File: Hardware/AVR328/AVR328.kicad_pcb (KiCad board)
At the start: 2 copper layers, 58.5 x 56.9 mm, 33 parts, among them J1 EJ508A, J2 284512-8, J3 284512-8, Q2 S9013, Q3 S9013, Q4 S9013, Q5 S9013, U1 ATMEGA328P-AU, U2 L78M05CDT, Y1 Crystal

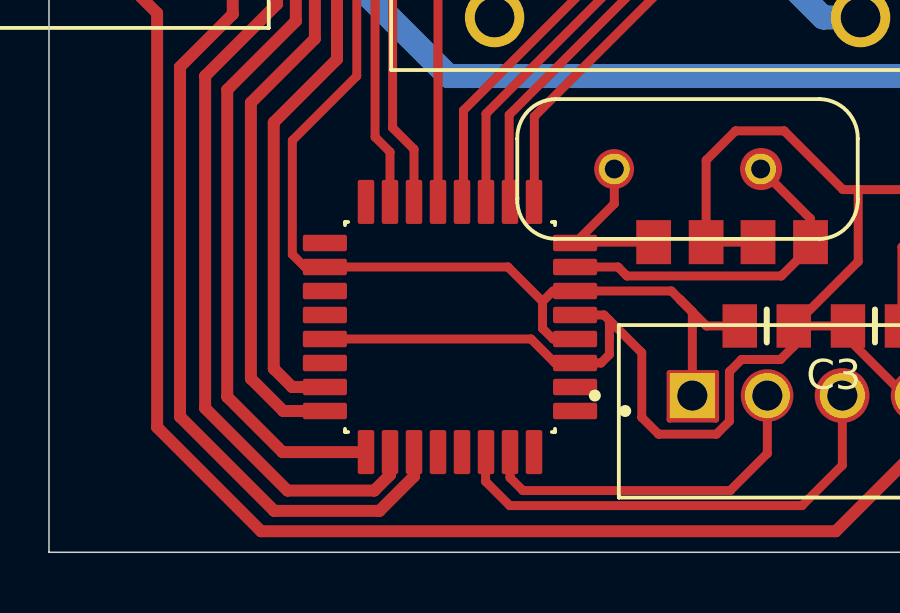
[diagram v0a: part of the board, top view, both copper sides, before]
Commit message: add
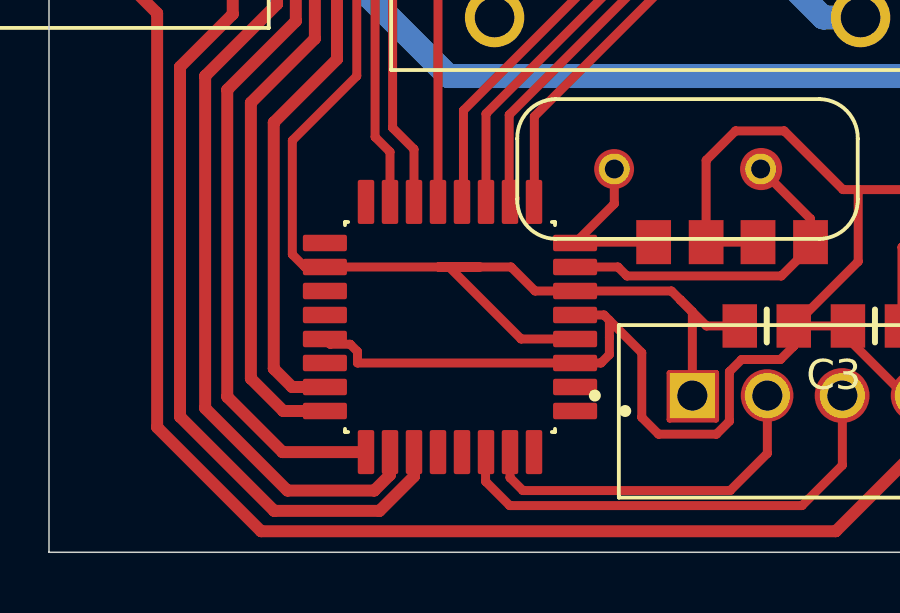
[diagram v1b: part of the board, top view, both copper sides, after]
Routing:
- net 5V: track 193.3 -> 197.5 mm
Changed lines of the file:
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@@
 		(tenting front back)
 		(pcbplotparams
-			(layerselection 0x00000000_00000000_55555555_555555f0)
+			(layerselection 0x00000000_00000000_55555555_55555554)
 			(plot_on_all_layers_selection 0x00000000_00000000_00000000_02000000)
 			(disableapertmacros no)
@@
 			(subtractmaskfromsilk no)
 			(outputformat 4)
-			(mirror no)
+			(mirror yes)
 			(drillshape 0)
 			(scaleselection 1)
@@
 	)
 	(segment
-		(start 73.931778 94.4652)
-		(end 74.731778 95.2652)
-		(width 0.3)
-		(layer "F.Cu")
-		(net 1)
-	)
-	(segment
 		(start 59.7017 81.8388)
 		(end 61.468 83.6051)
@@
 	)
 	(segment
+		(start 68.1458 95.2652)
+		(end 75.3998 95.2652)
+		(width 0.3)
+		(layer "F.Cu")
+		(net 1)
+	)
+	(segment
 		(start 100.2507 89.4854)
 		(end 100.47 89.7047)
@@
 	)
 	(segment
+		(start 67.901822 94.6392)
+		(end 68.1458 94.883178)
+		(width 0.3)
+		(layer "F.Cu")
+		(net 1)
+	)
+	(segment
 		(start 84.3292 89.4854)
 		(end 82.3722 87.5284)
@@
 	)
 	(segment
-		(start 67.0598 94.4652)
-		(end 73.931778 94.4652)
-		(width 0.3)
-		(layer "F.Cu")
-		(net 1)
-	)
-	(segment
 		(start 94.2848 89.4854)
 		(end 94.2848 89.4588)
@@
 	)
 	(segment
-		(start 75.3998 93.6652)
-		(end 76.365 93.6652)
+		(start 67.0598 94.4652)
+		(end 67.2338 94.6392)
 		(width 0.3)
 		(layer "F.Cu")
@@
 	)
 	(segment
-		(start 94.2848 89.4854)
-		(end 100.2507 89.4854)
+		(start 75.3998 93.6652)
+		(end 76.365 93.6652)
 		(width 0.3)
 		(layer "F.Cu")
@@
 	)
 	(segment
-		(start 74.731778 95.2652)
-		(end 75.3998 95.2652)
+		(start 94.2848 89.4854)
+		(end 100.2507 89.4854)
 		(width 0.3)
 		(layer "F.Cu")
@@
 	)
 	(segment
+		(start 68.1458 94.883178)
+		(end 68.1458 95.2652)
+		(width 0.3)
+		(layer "F.Cu")
+		(net 1)
+	)
+	(segment
 		(start 95.9612 64.8028)
 		(end 95.9612 53.6956)
@@
 	)
 	(segment
+		(start 67.2338 94.6392)
+		(end 67.901822 94.6392)
+		(width 0.3)
+		(layer "F.Cu")
+		(net 1)
+	)
+	(segment
 		(start 76.8288 92.0652)
 		(end 77.1278 92.3642)
@@
 	)
 	(segment
-		(start 73.1628 92.0652)
-		(end 74.3138 93.2162)
-		(width 0.3)
-		(layer "F.Cu")
-		(net 5)
-	)
-	(segment
 		(start 72.7162 71.7494)
 		(end 74.6196 71.7494)
@@
 	)
 	(segment
+		(start 67.0598 92.0652)
+		(end 70.85 92.0652)
+		(width 0.3)
+		(layer "F.Cu")
+		(net 5)
+	)
+	(segment
+		(start 74.0652 92.8652)
+		(end 75.3998 92.8652)
+		(width 0.3)
+		(layer "F.Cu")
+		(net 5)
+	)
+	(segment
 		(start 107.1118 72.3392)
 		(end 107.1118 65.2526)
@@
 	)
 	(segment
+		(start 73.2652 92.0652)
+		(end 74.0652 92.8652)
+		(width 0.3)
+		(layer "F.Cu")
+		(net 5)
+	)
+	(segment
 		(start 62.6812 55.632)
 		(end 72.7314 55.632)
@@
 	)
 	(segment
+		(start 73.6 94.4652)
+		(end 71.2 92.0652)
+		(width 0.3)
+		(layer "F.Cu")
+		(net 5)
+	)
+	(segment
 		(start 72.7314 55.632)
 		(end 74.4668 55.632)
@@
 	)
 	(segment
-		(start 74.6648 94.4652)
-		(end 75.3998 94.4652)
+		(start 75.3998 94.4652)
+		(end 73.6 94.4652)
 		(width 0.3)
 		(layer "F.Cu")
@@
 	)
 	(segment
-		(start 74.6648 92.8652)
-		(end 74.3138 93.2162)
-		(width 0.3)
-		(layer "F.Cu")
-		(net 5)
-	)
-	(segment
 		(start 104.5835 83.7494)
 		(end 103.9114 83.0773)
@@
 	)
 	(segment
-		(start 74.3138 93.2162)
-		(end 74.3138 94.1142)
+		(start 107.1118 65.2526)
+		(end 104.0638 62.2046)
 		(width 0.3)
 		(layer "F.Cu")
@@
 	)
 	(segment
-		(start 107.1118 65.2526)
-		(end 104.0638 62.2046)
+		(start 72.240298 92.0652)
+		(end 70.85 92.0652)
 		(width 0.3)
 		(layer "F.Cu")
@@
 	)
 	(segment
-		(start 75.3998 92.8652)
-		(end 74.6648 92.8652)
-		(width 0.3)
-		(layer "F.Cu")
-		(net 5)
-	)
-	(segment
 		(start 65.9738 87.8486)
 		(end 68.1228 85.6996)
@@
 	)
 	(segment
-		(start 74.3138 94.1142)
-		(end 74.6648 94.4652)
-		(width 0.3)
-		(layer "F.Cu")
-		(net 5)
-	)
-	(segment
 		(start 78.9037 93.1559)
 		(end 78.613 92.8652)
@@
 	)
 	(segment
-		(start 67.0598 92.0652)
-		(end 73.1628 92.0652)
+		(start 106.3752 54.356)
+		(end 105.918 53.8988)
 		(width 0.3)
 		(layer "F.Cu")
@@
 	)
 	(segment
-		(start 106.3752 54.356)
-		(end 105.918 53.8988)
+		(start 71.2 92.0652)
+		(end 73.2652 92.0652)
 		(width 0.3)
 		(layer "F.Cu")
@@
 		(layer "F.Cu")
 		(net 5)
+	)
+	(segment
+		(start 70.85 92.0652)
+		(end 71.2 92.0652)
+		(width 0.3)
+		(layer "F.Cu")
+		(net 5)

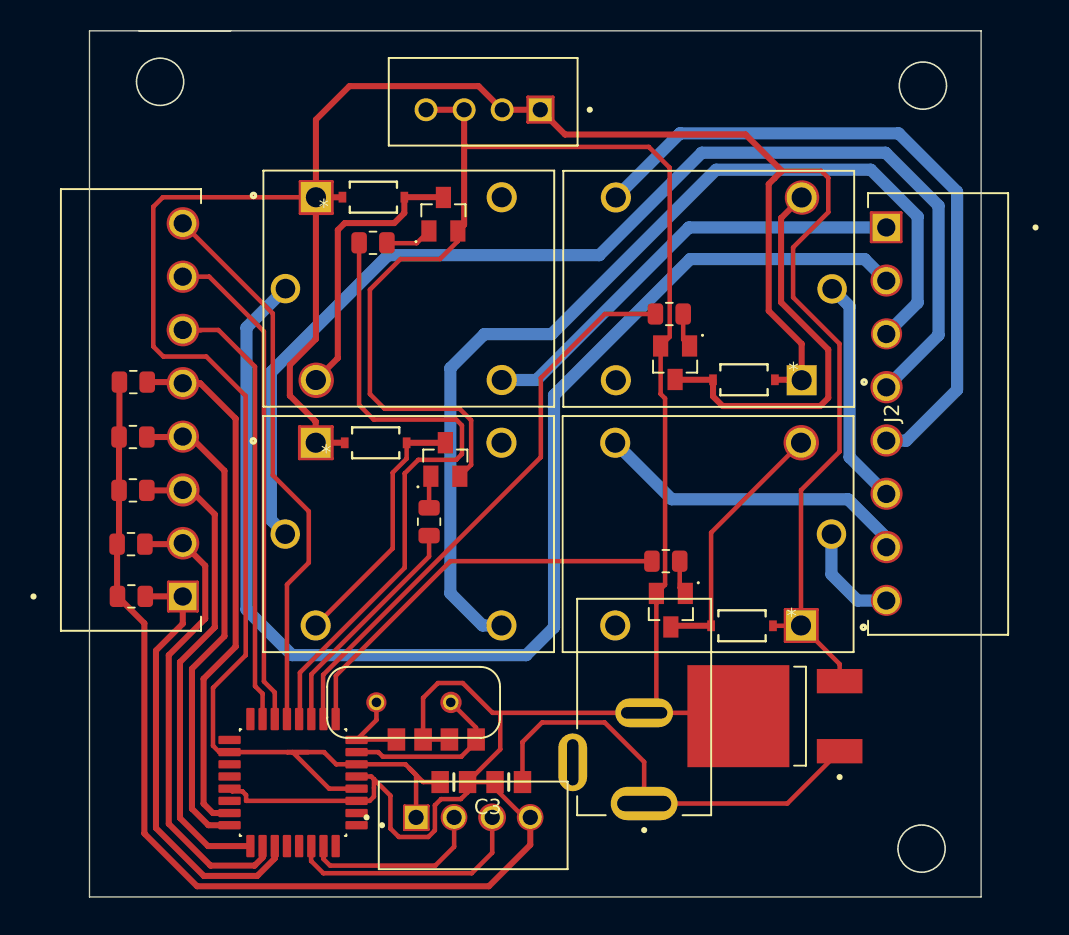
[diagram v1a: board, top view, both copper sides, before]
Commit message: add
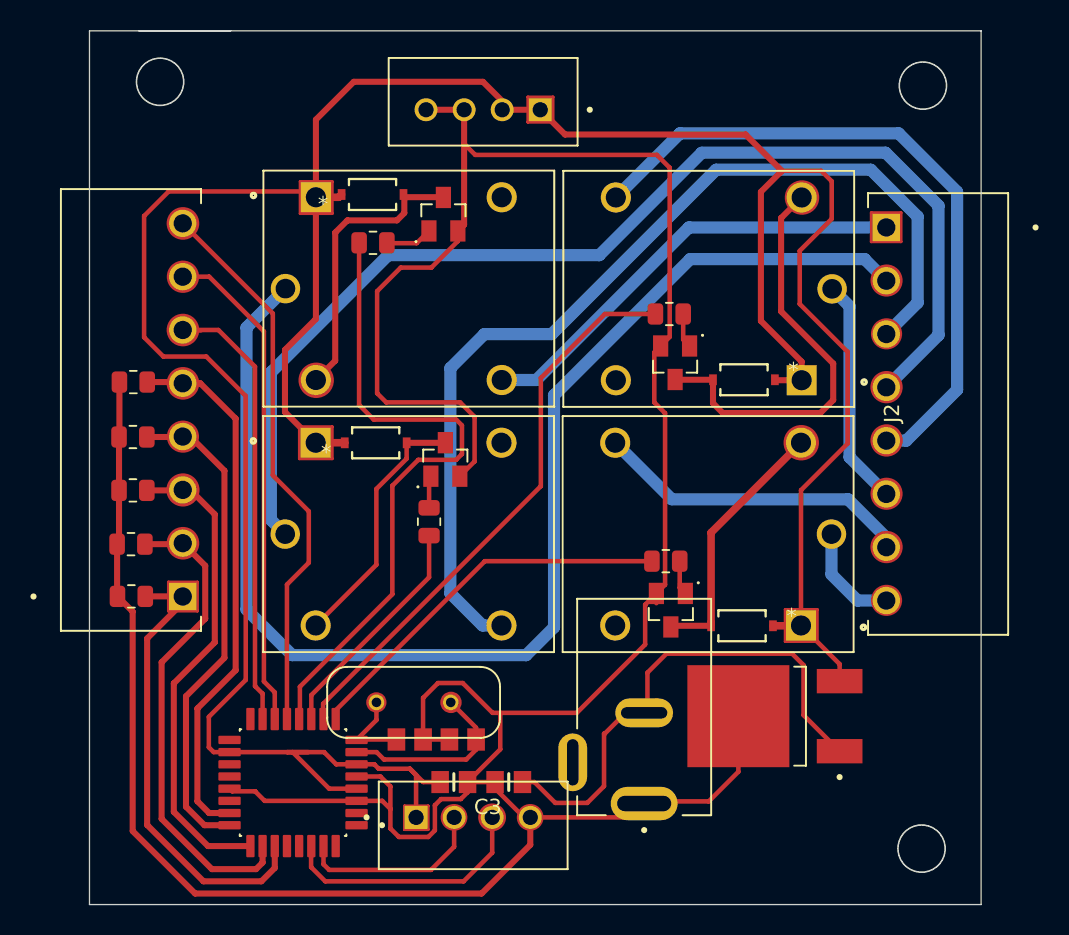
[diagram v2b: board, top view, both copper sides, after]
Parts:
- moved D1 0.18 mm to (76.5, 55.5)
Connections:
- J1 pad 1: Net-(U2-IN) -> GND
- J1 pad 2: GND -> Net-(U2-IN)
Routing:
- net GND: track 210.2 -> 221.0 mm
- net Net-(U2-IN): track 29.2 -> 34.6 mm
- net 5V: track 197.5 -> 200.4 mm
- net ADC0: track 29.8 -> 31.1 mm
- net OUT1: track 26.7 -> 25.4 mm
- net Net-(D3-A): track 26.7 -> 27.9 mm
- net ADC1: track 30.8 -> 31.7 mm
- net USART_RX: track 16.8 -> 17.4 mm
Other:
- board size 58.5 x 56.9 mm -> 58.5 x 57.4 mm
